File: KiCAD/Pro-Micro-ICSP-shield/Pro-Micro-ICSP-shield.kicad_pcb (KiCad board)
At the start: 2 copper layers, 33 x 17.8 mm, 14 parts, among them J1 Pro Micro, J2 ICSP, SW1 MODE, SW2 RESET

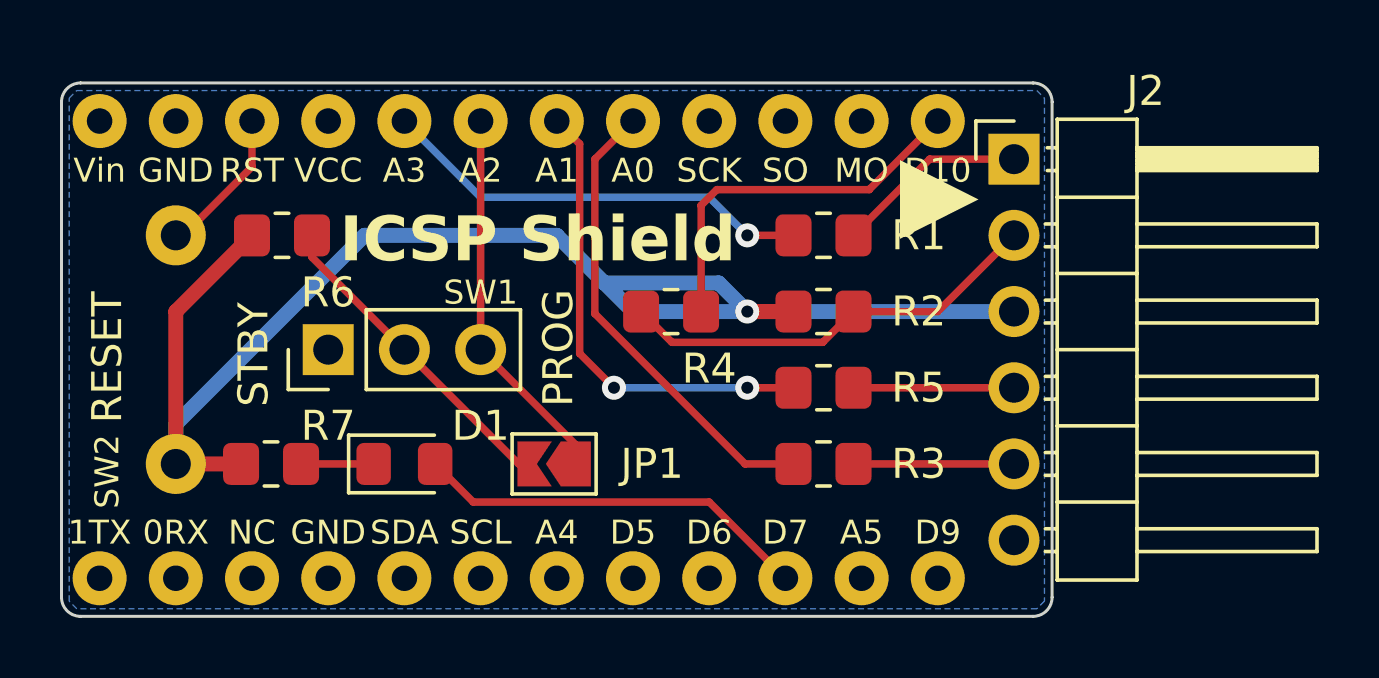
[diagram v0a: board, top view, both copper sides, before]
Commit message: Add Pro-Micro-ICSP-shield-1.1
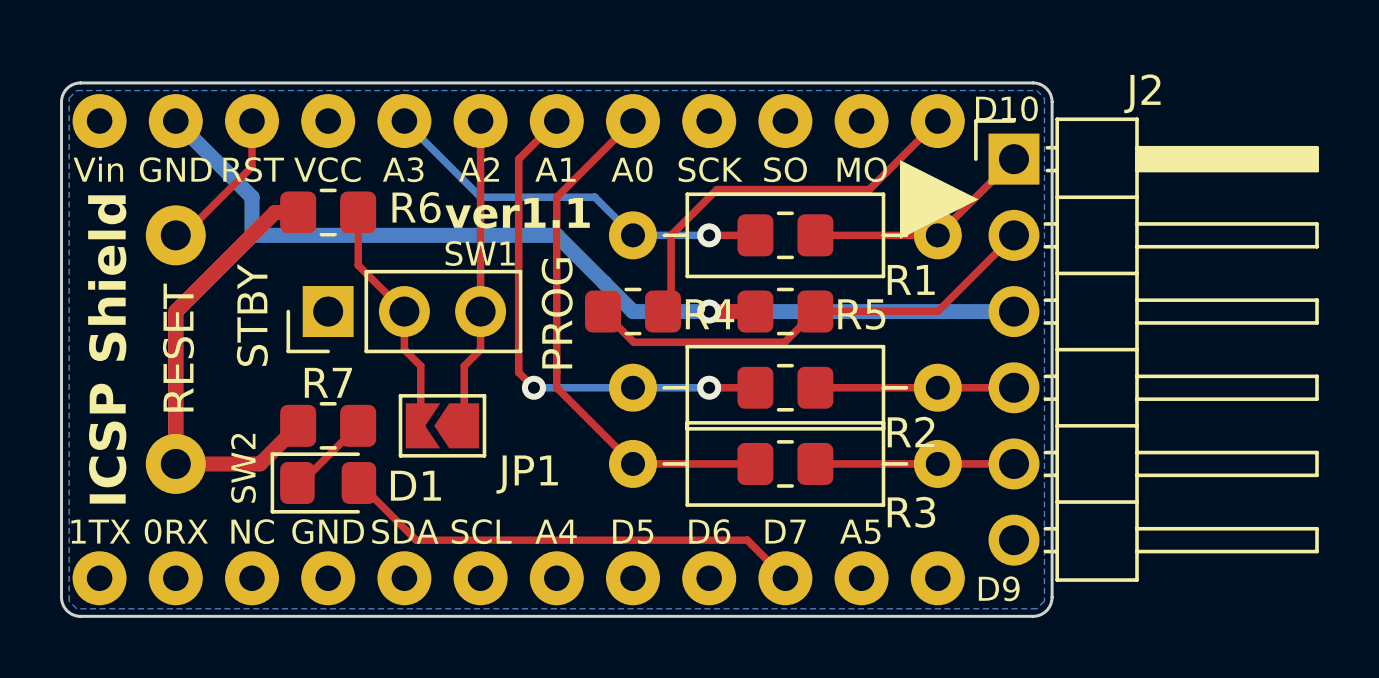
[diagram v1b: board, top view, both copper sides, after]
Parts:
- added R10: 470, Resistor_THT:R_Axial_DIN0207_L6.3mm_D2.5mm_P10.16mm_Horizontal, F.Cu at (156.2, 97.8)
- added R8: 470, Resistor_THT:R_Axial_DIN0207_L6.3mm_D2.5mm_P10.16mm_Horizontal, F.Cu at (156.2, 105.4)
- added R9: 470, Resistor_THT:R_Axial_DIN0207_L6.3mm_D2.5mm_P10.16mm_Horizontal, F.Cu at (156.2, 102.9)
- moved JP1 3.93 mm to (149.9, 104.1)
- moved D1 2.62 mm to (146.1, 106.0)
- moved R7 2.29 mm to (146.1, 104.1)
- moved R6 1.72 mm to (146.1, 97.0)
- moved R1 1.27 mm to (161.3, 97.8)
- moved R2 1.27 mm to (161.3, 102.9)
- moved R3 1.27 mm to (161.3, 105.4)
- moved R5 1.27 mm to (161.3, 100.3)
- moved SW1 1.27 mm to (146.1, 100.3)
- moved R4 1.27 mm to (156.2, 100.3)
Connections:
- net Net-(J1-D14/A0) renamed A0
- net Net-(J1-D15/A1) renamed A1
- net Net-(J1-D18/A3) renamed A3
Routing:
- net GND: track 50.5 -> 56.7 mm
- net Net-(JP1-B): track 10.9 -> 7.98 mm
- net PROG: track 12.7 -> 10.4 mm
- net LED: track 13.3 -> 15.5 mm
- net A0: track 15.6 -> 17.6 mm
- net A1: track 15.7 -> 17.0 mm
- net A3: track 14.5 -> 13.3 mm
- net PGD: track 5.35 -> 6.62 mm
- net PGC: track 5.35 -> 6.62 mm
- net MCLR: track 6.40 -> 7.67 mm
- net VDD: track 14.3 -> 15.6 mm
- net Net-(J1-D10/A10): track 12.6 -> 13.1 mm
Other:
- board text added: "@hanyazou June 4, 2023"
- board text added: "ICSP Shield Rev 1.1"
- board text added: "ver1.1"
- board text removed: "@hanyazou Mar 18, 2023"
- board text removed: "ICSP Shield Rev 1.0"
